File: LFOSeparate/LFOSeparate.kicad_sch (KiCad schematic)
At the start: 31 parts, among them IC1 PIC16F15325-I_P, IC2 MCP6232-E_P, IC3 MCP6232-E_P, J1 ICSP, J2 D_Power, J3 Input, J4 Output, J5 A_Power, U1 Opamp_Dual

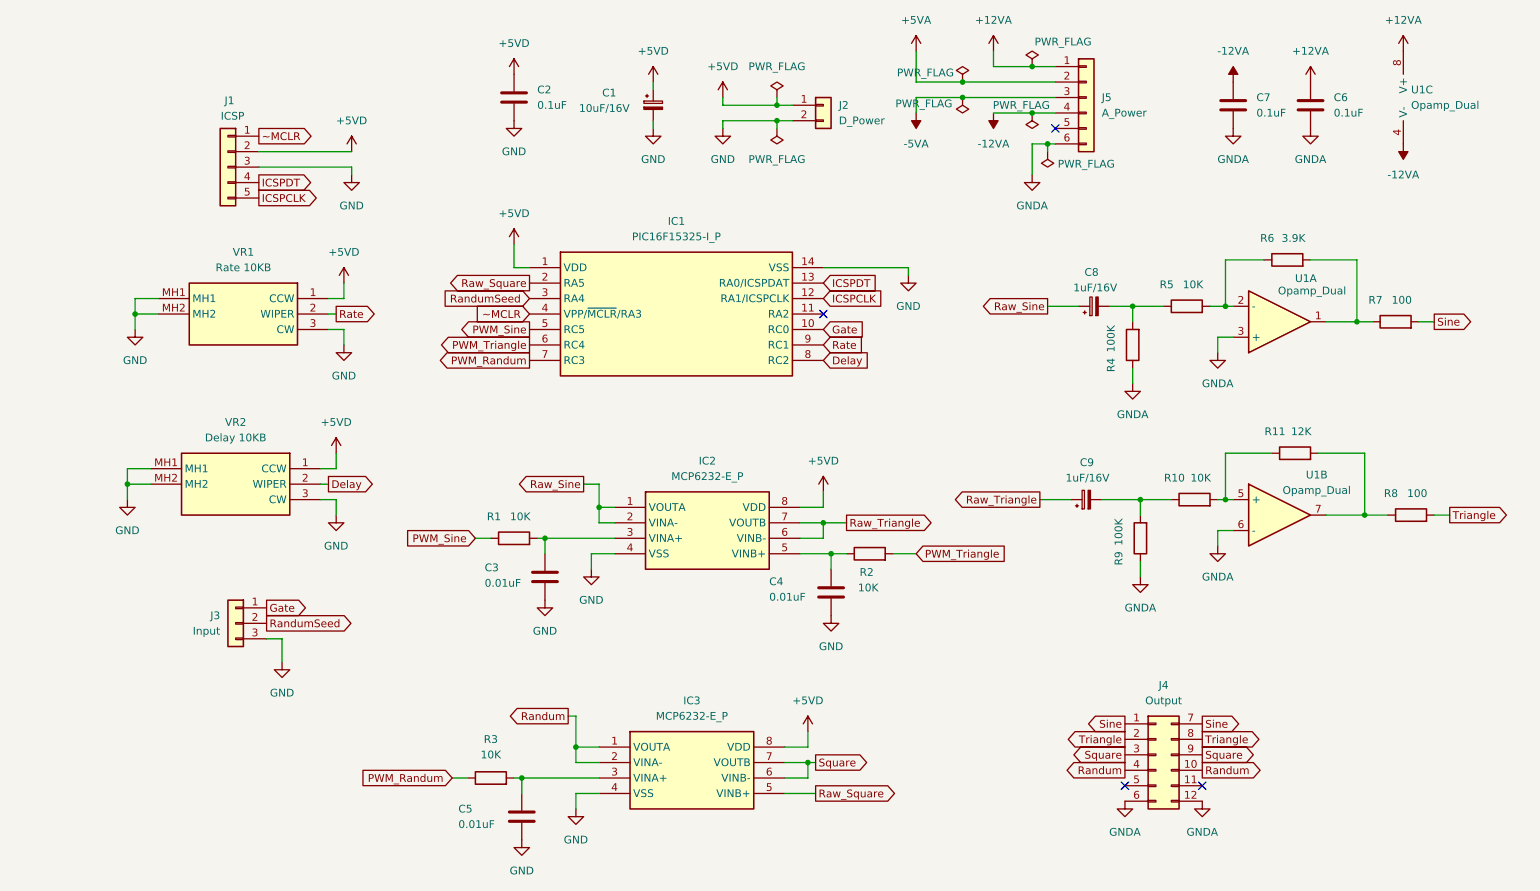
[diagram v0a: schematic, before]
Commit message: LFOSeparate
アートワーク作成中
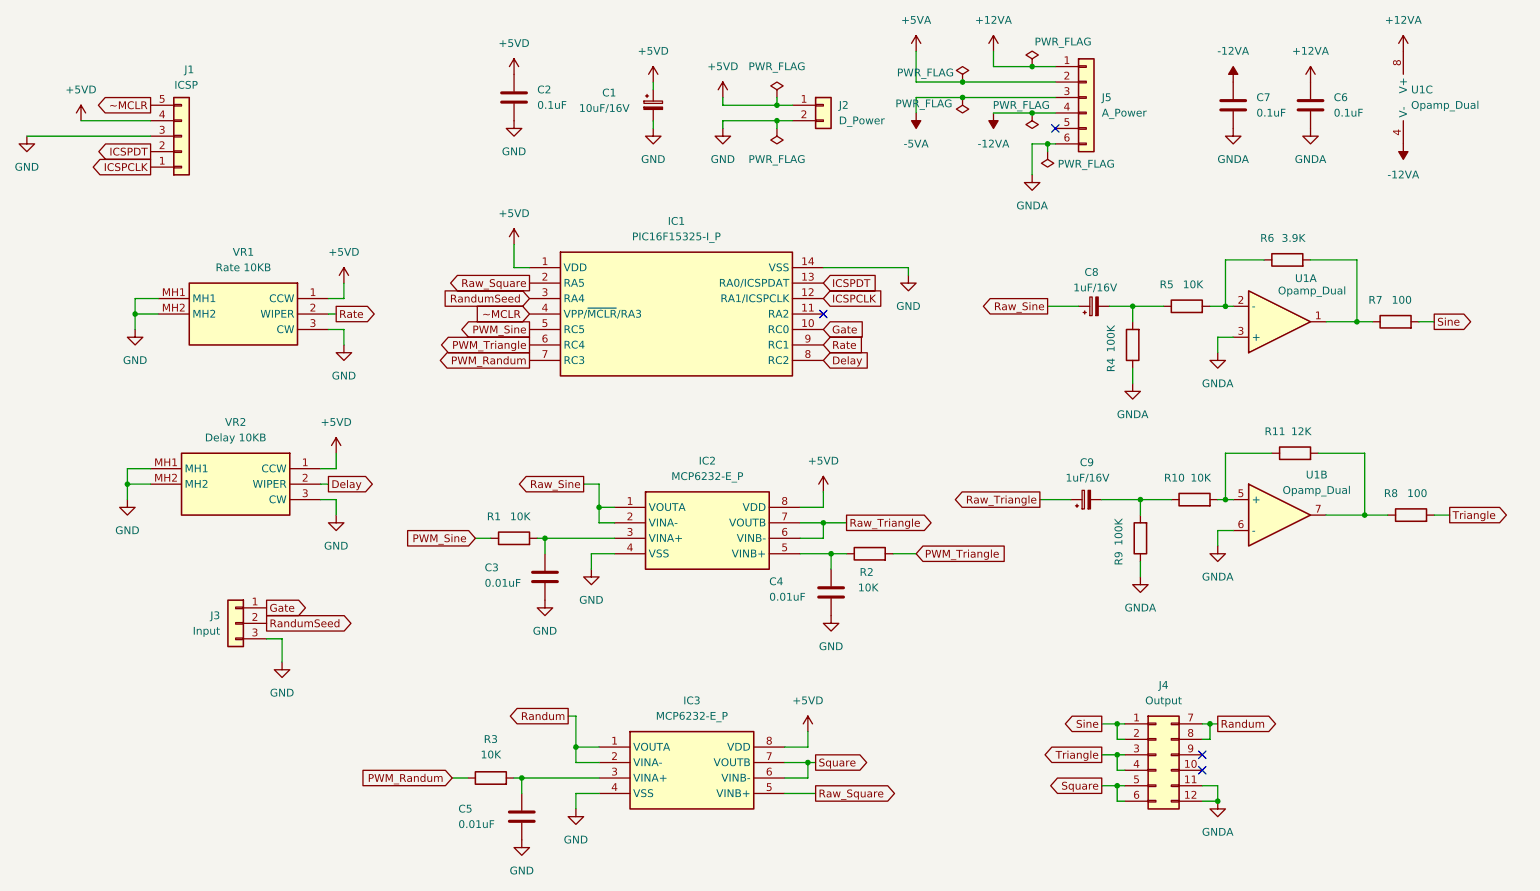
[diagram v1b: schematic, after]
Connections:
- net +5VD: now also J1.4 (Pin_4); no longer J1.2 (Pin_2)
- net GNDA: now also J4.11 (Pin_11); no longer J4.6 (Pin_6)
- net ICSPCLK: now also J1.1 (Pin_1); no longer J1.5 (Pin_5)
- net ICSPDT: now also J1.2 (Pin_2); no longer J1.4 (Pin_4)
- net Randum: now also J4.7 (Pin_7), J4.8 (Pin_8); no longer J4.10 (Pin_10), J4.4 (Pin_4)
- net Sine: now also J4.2 (Pin_2); no longer J4.7 (Pin_7)
- net Square: now also J4.5 (Pin_5), J4.6 (Pin_6); no longer J4.3 (Pin_3), J4.9 (Pin_9)
- net Triangle: now also J4.3 (Pin_3), J4.4 (Pin_4); no longer J4.2 (Pin_2), J4.8 (Pin_8)
- net ~MCLR: now also J1.5 (Pin_5); no longer J1.1 (Pin_1)
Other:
- moved on the sheet: J1
